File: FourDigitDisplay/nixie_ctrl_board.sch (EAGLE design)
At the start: 23 parts, among them CN1 PIC_CN_H, CN2 I2C_IF, Q1 IN-12B, Q2 IN-12B, Q3 IN-12B, Q4 IN-12B, U1 TLP627-2, U2 SN74141, U3 TLP627-2, U4 SN74141, U5 PIC16F18857-I/SP

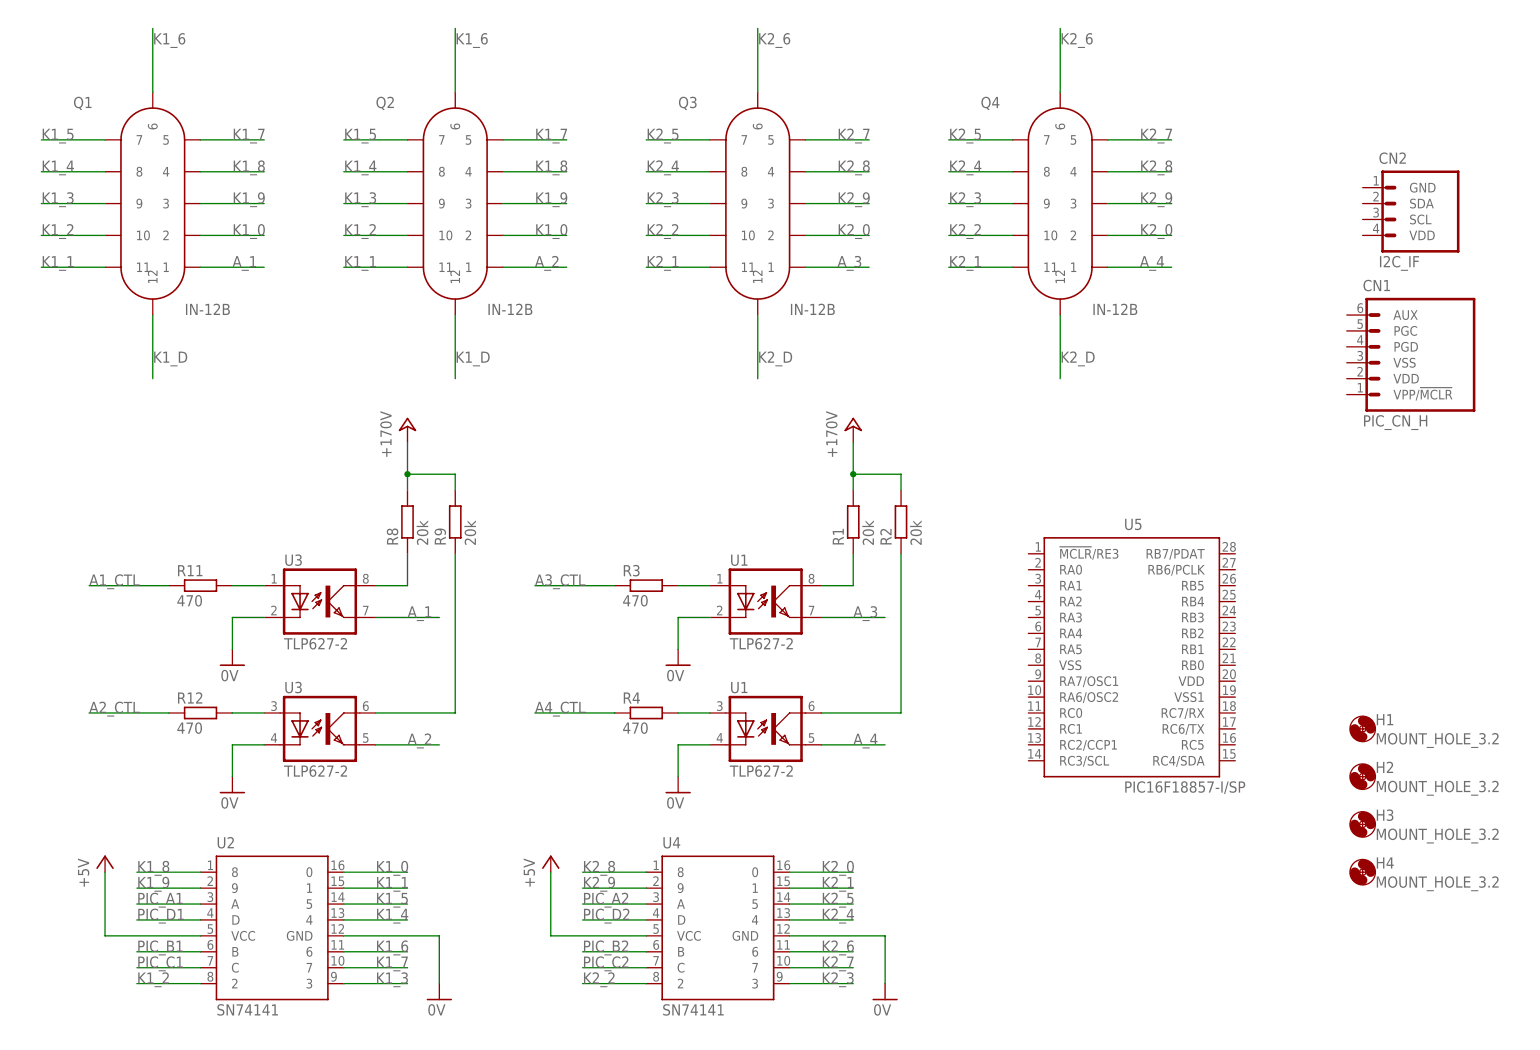
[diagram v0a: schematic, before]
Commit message: 配線の追加
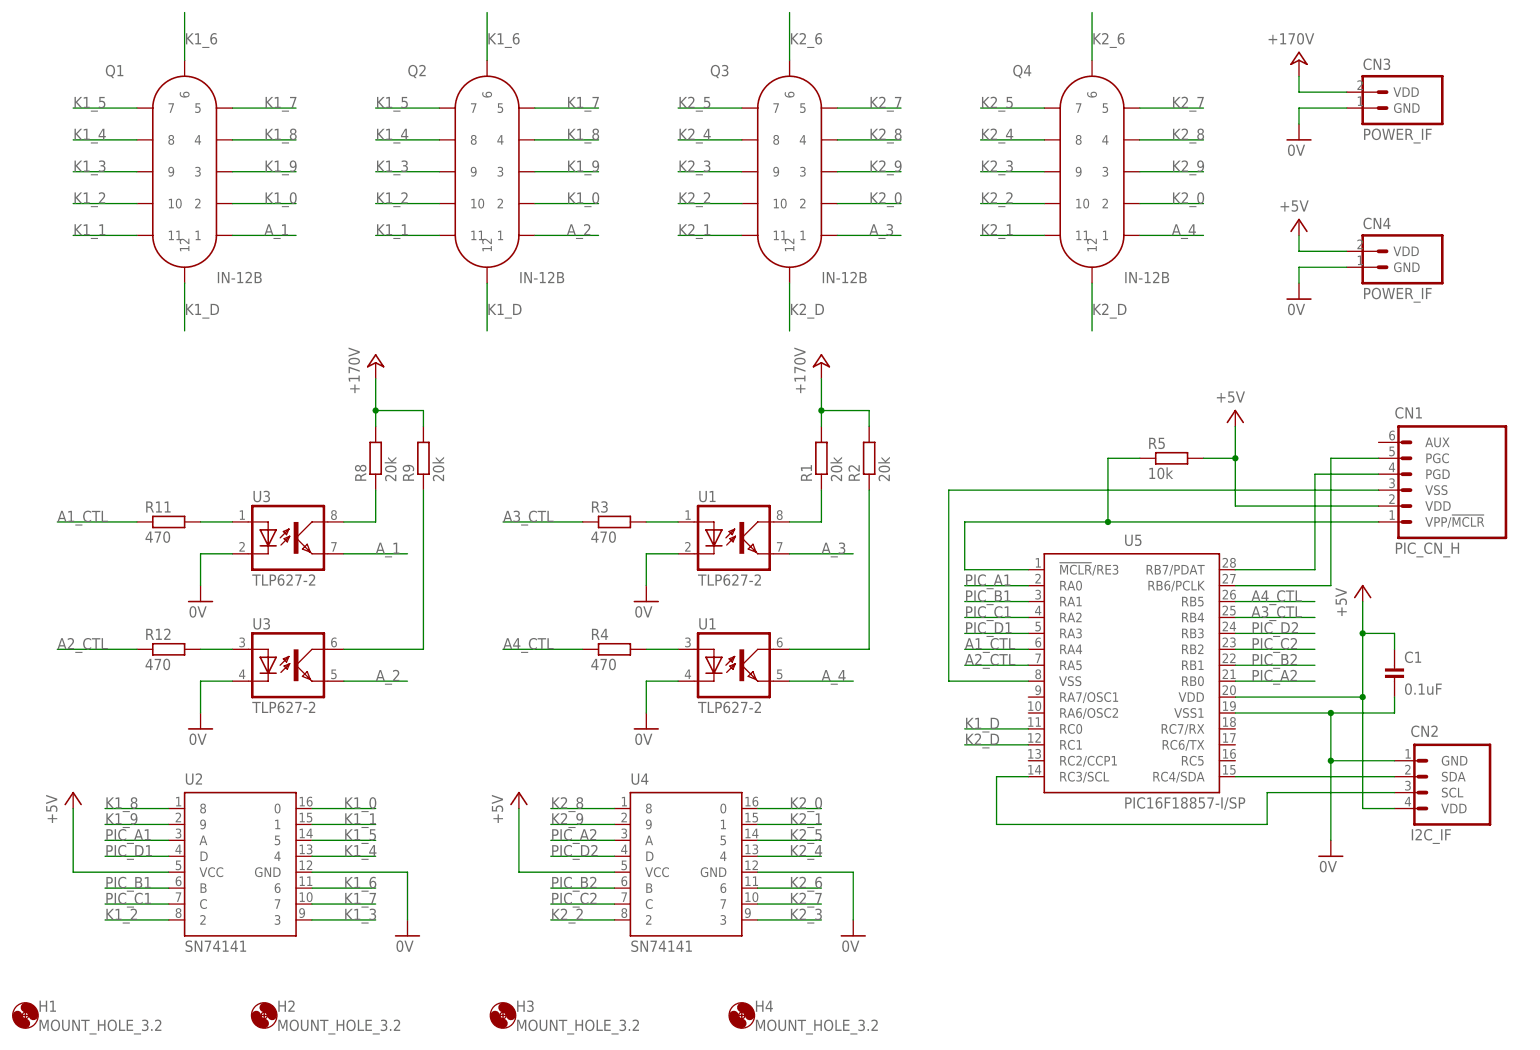
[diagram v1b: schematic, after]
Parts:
- added C1: 0.1uF, Parts:CAP_100MIL
- added CN3, CN4: POWER_IF, PartsForProto:POWER_IF
- added R5: 10k, Parts:RESISTOR_300MIL
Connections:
- new net N$15: CN1.VSS, U5.VSS
- new net N$5: CN2.SDA, U5.RC4/SDA
- new net N$6: CN2.SCL, U5.RC3/SCL
- new net N$7: CN1.VPP/!MCLR, R5.1, U5.!MCLR!/RE3
- new net N$8: CN1.PGD, U5.RB7/PDAT
- new net N$9: CN1.PGC, U5.RB6/PCLK
- net +24V: now also CN3.VDD
- net +5V: now also C1.1, CN1.VDD, CN2.VDD, CN4.VDD, R5.2, U5.VDD
- net 0V: now also C1.2, CN2.GND, CN3.GND, CN4.GND, U5.VSS1
- net A1_CTL: now also U5.RA4
- net A2_CTL: now also U5.RA5
- net A3_CTL: now also U5.RB4
- net A4_CTL: now also U5.RB5
- net K1_D: now also U5.RC0
- net K2_D: now also U5.RC1
- net PIC_A1: now also U5.RA0
- net PIC_A2: now also U5.RB0
- net PIC_B1: now also U5.RA1
- net PIC_B2: now also U5.RB1
- net PIC_C1: now also U5.RA2
- net PIC_C2: now also U5.RB2
- net PIC_D1: now also U5.RA3
- net PIC_D2: now also U5.RB3
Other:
- moved on the sheet: CN1, CN2, H1, H2, H3, H4, Q1, Q2, Q3, Q4, R1, R11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
